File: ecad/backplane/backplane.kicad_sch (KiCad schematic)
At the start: 18 parts, among them J1 10145891-0320J13LF, J2 10145891-0320J13LF, J3 10145891-0320J13LF, J4 10145891-0320J13LF, J6 USB4105-GF-A, U1 MCP16331x-xCH

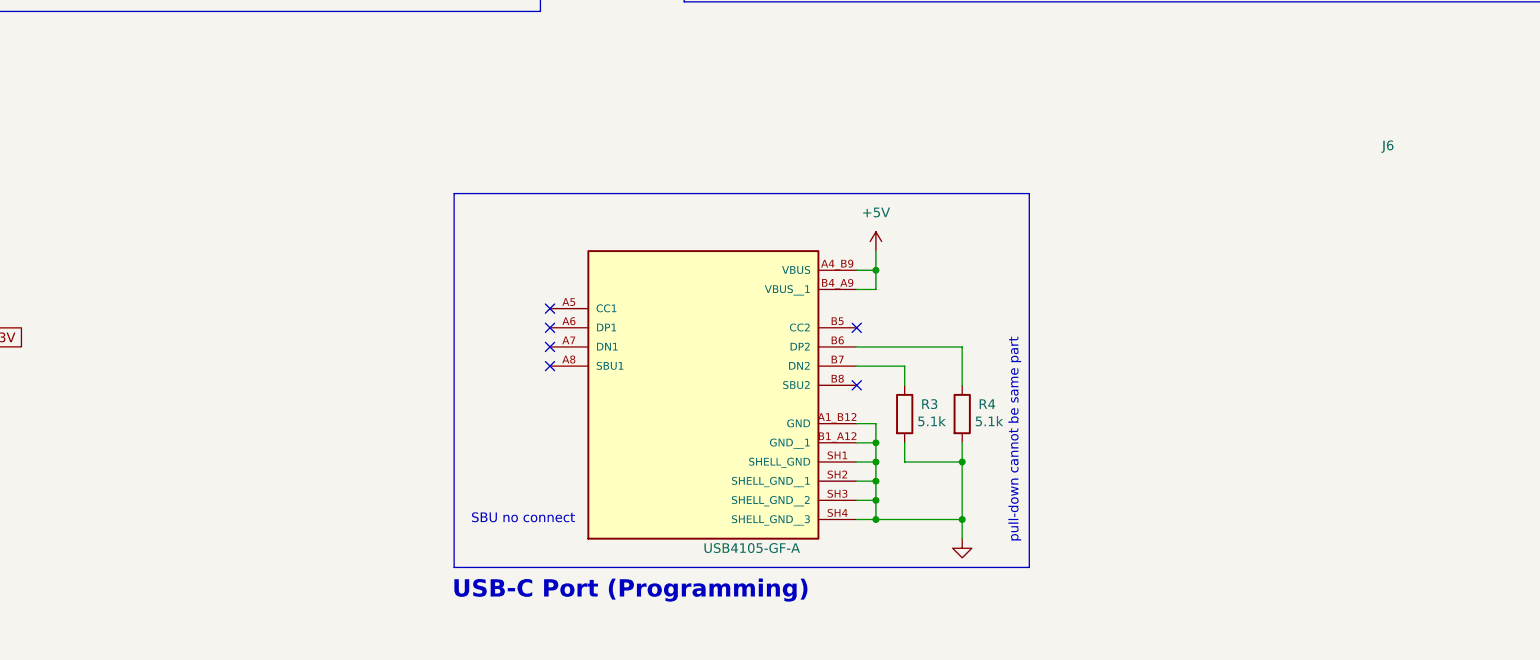
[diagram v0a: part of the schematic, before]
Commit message: hii
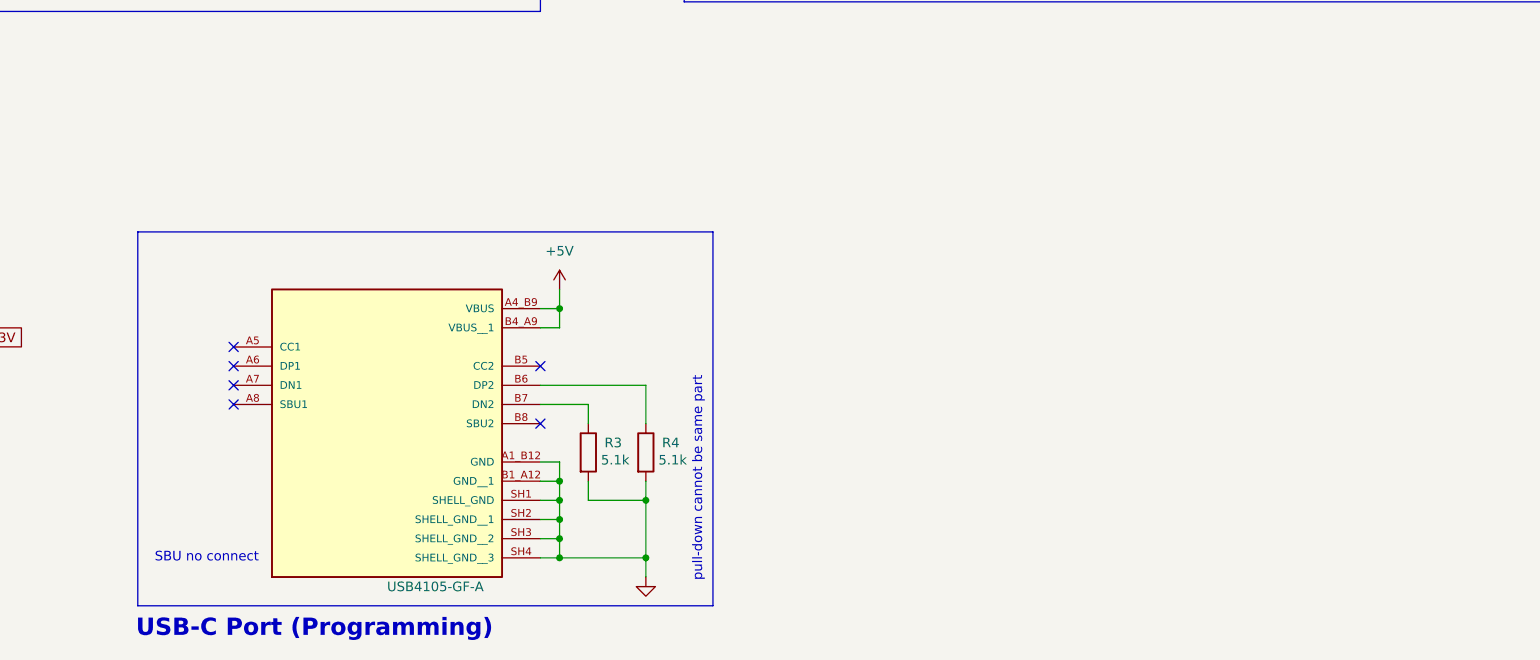
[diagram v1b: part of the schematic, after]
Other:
- moved on the sheet: R3, R4
